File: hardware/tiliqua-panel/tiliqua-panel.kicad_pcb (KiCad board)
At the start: 2 copper layers, 30 x 128.5 mm, 13 parts

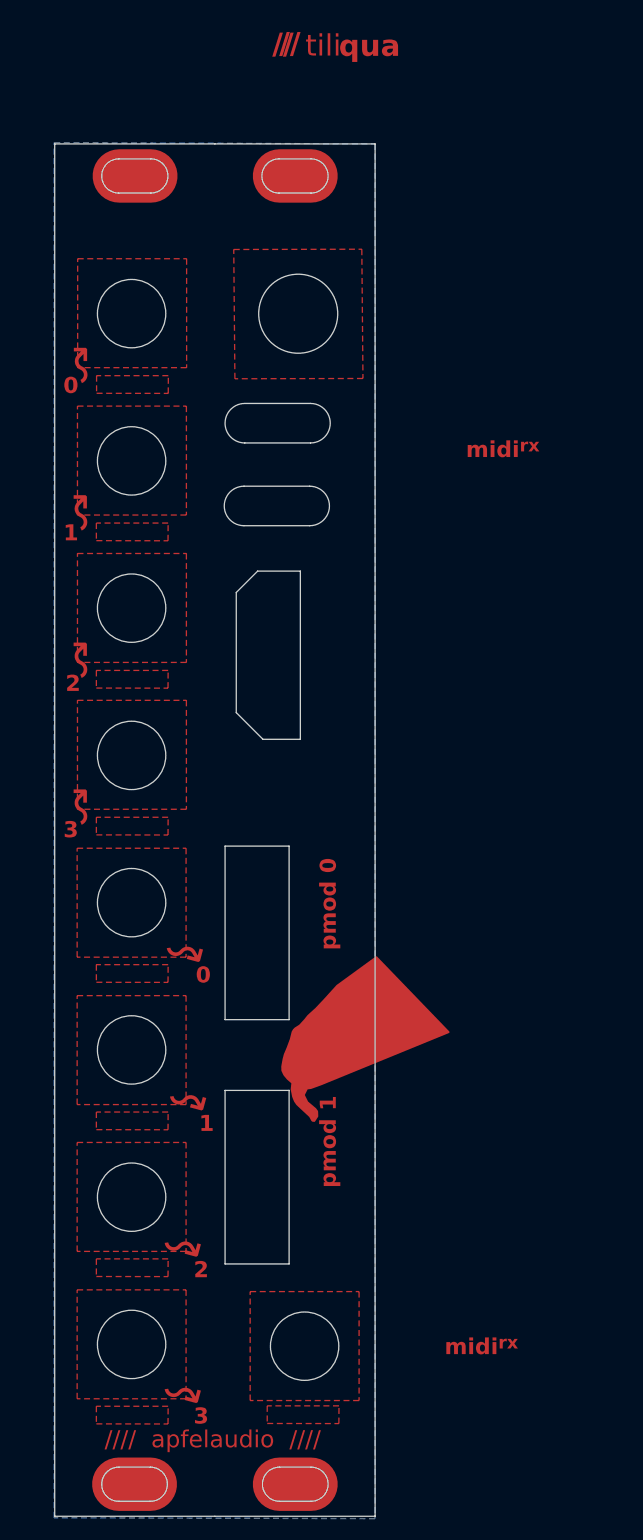
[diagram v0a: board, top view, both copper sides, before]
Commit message: panel jumble
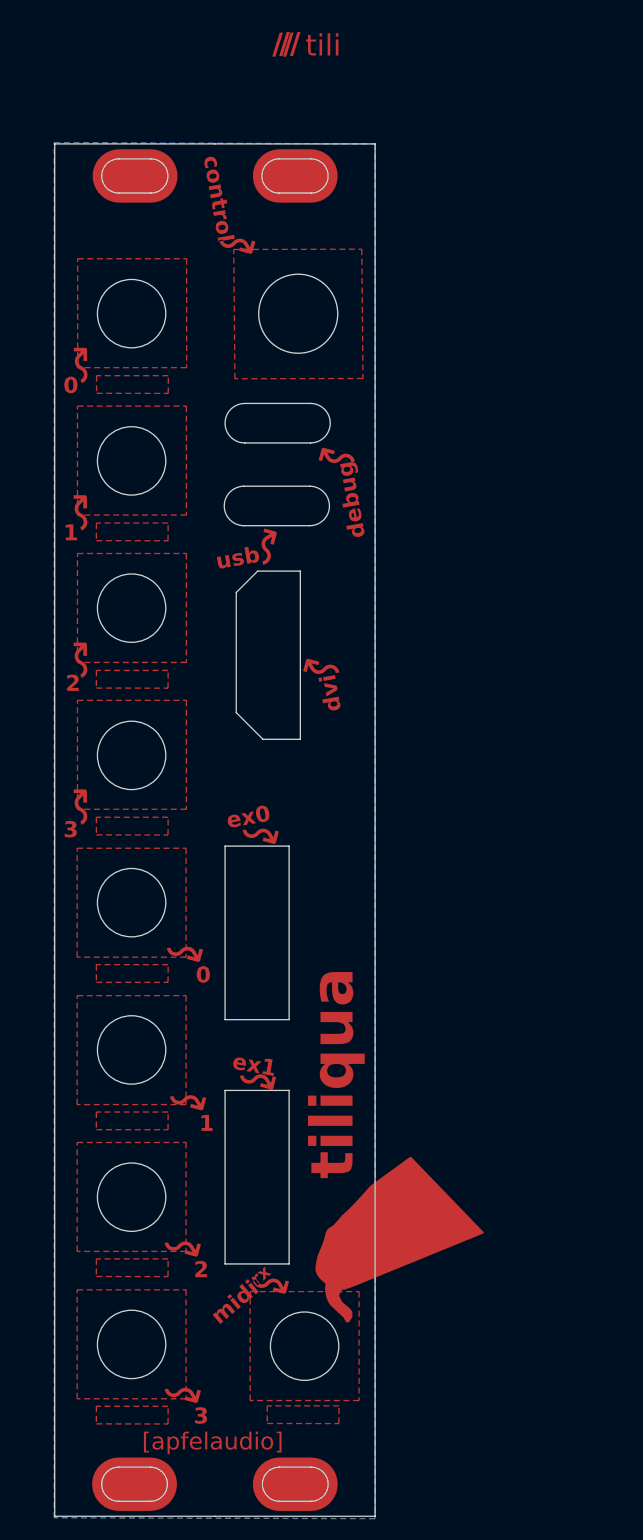
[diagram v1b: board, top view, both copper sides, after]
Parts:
- moved G*** 19.0 mm to (26.8, 103.3)
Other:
- board text added: "[apfelaudio]"
- board text added: "control"
- board text added: "debug"
- board text added: "dvi"
- board text added: "ex0"
- board text added: "ex1"
- board text added: "tiliqua"
- board text added: "usb"
- board text removed: "//// apfelaudio ////"
- board text removed: "pmod 0"
- board text removed: "pmod 1"
